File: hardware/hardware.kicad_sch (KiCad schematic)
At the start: 30 parts, among them J2 AudioPlug4, J3 USB_C_Receptacle_USB2.0, J4 AudioPlug4, SW1 SW_Push, SW2 SW_Push, SW3 SW_Push, SW4 SW_Push, SW5 SW_Push, SW6 SW_Push, SW7 SW_Push

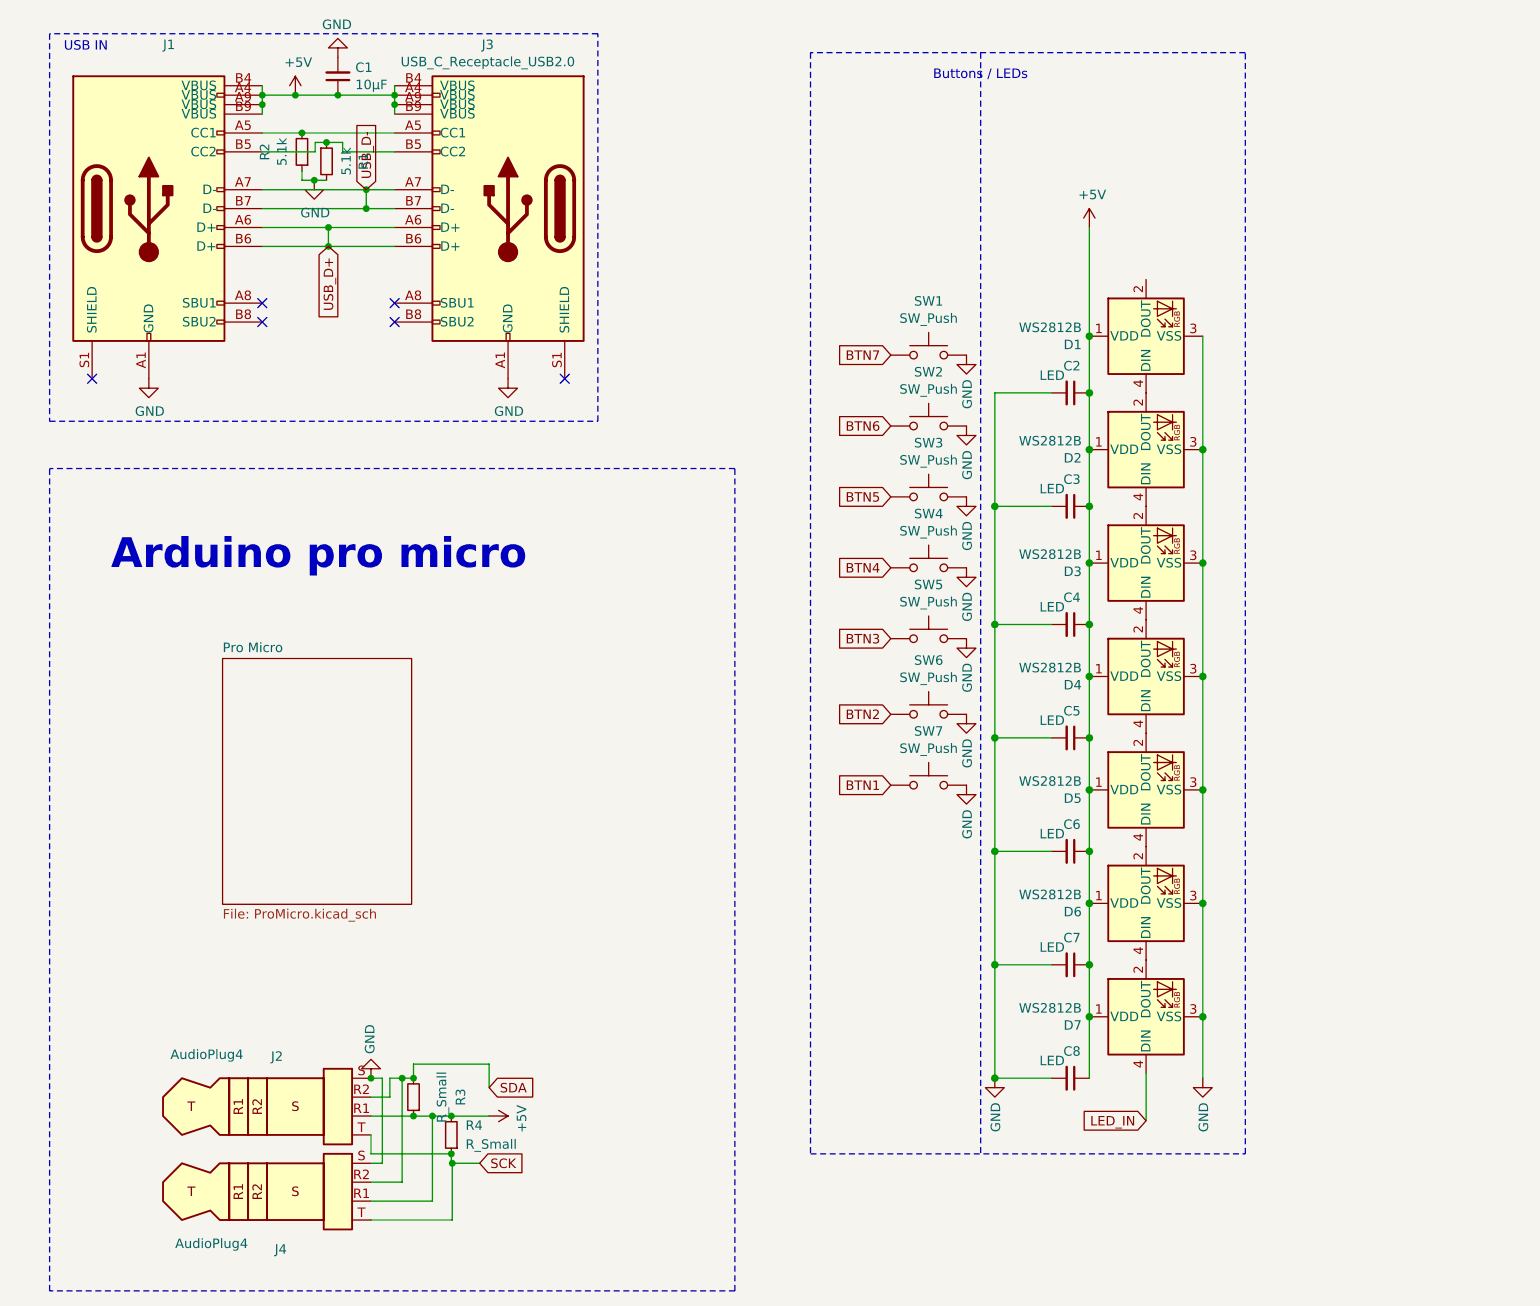
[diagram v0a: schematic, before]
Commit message: finish routing
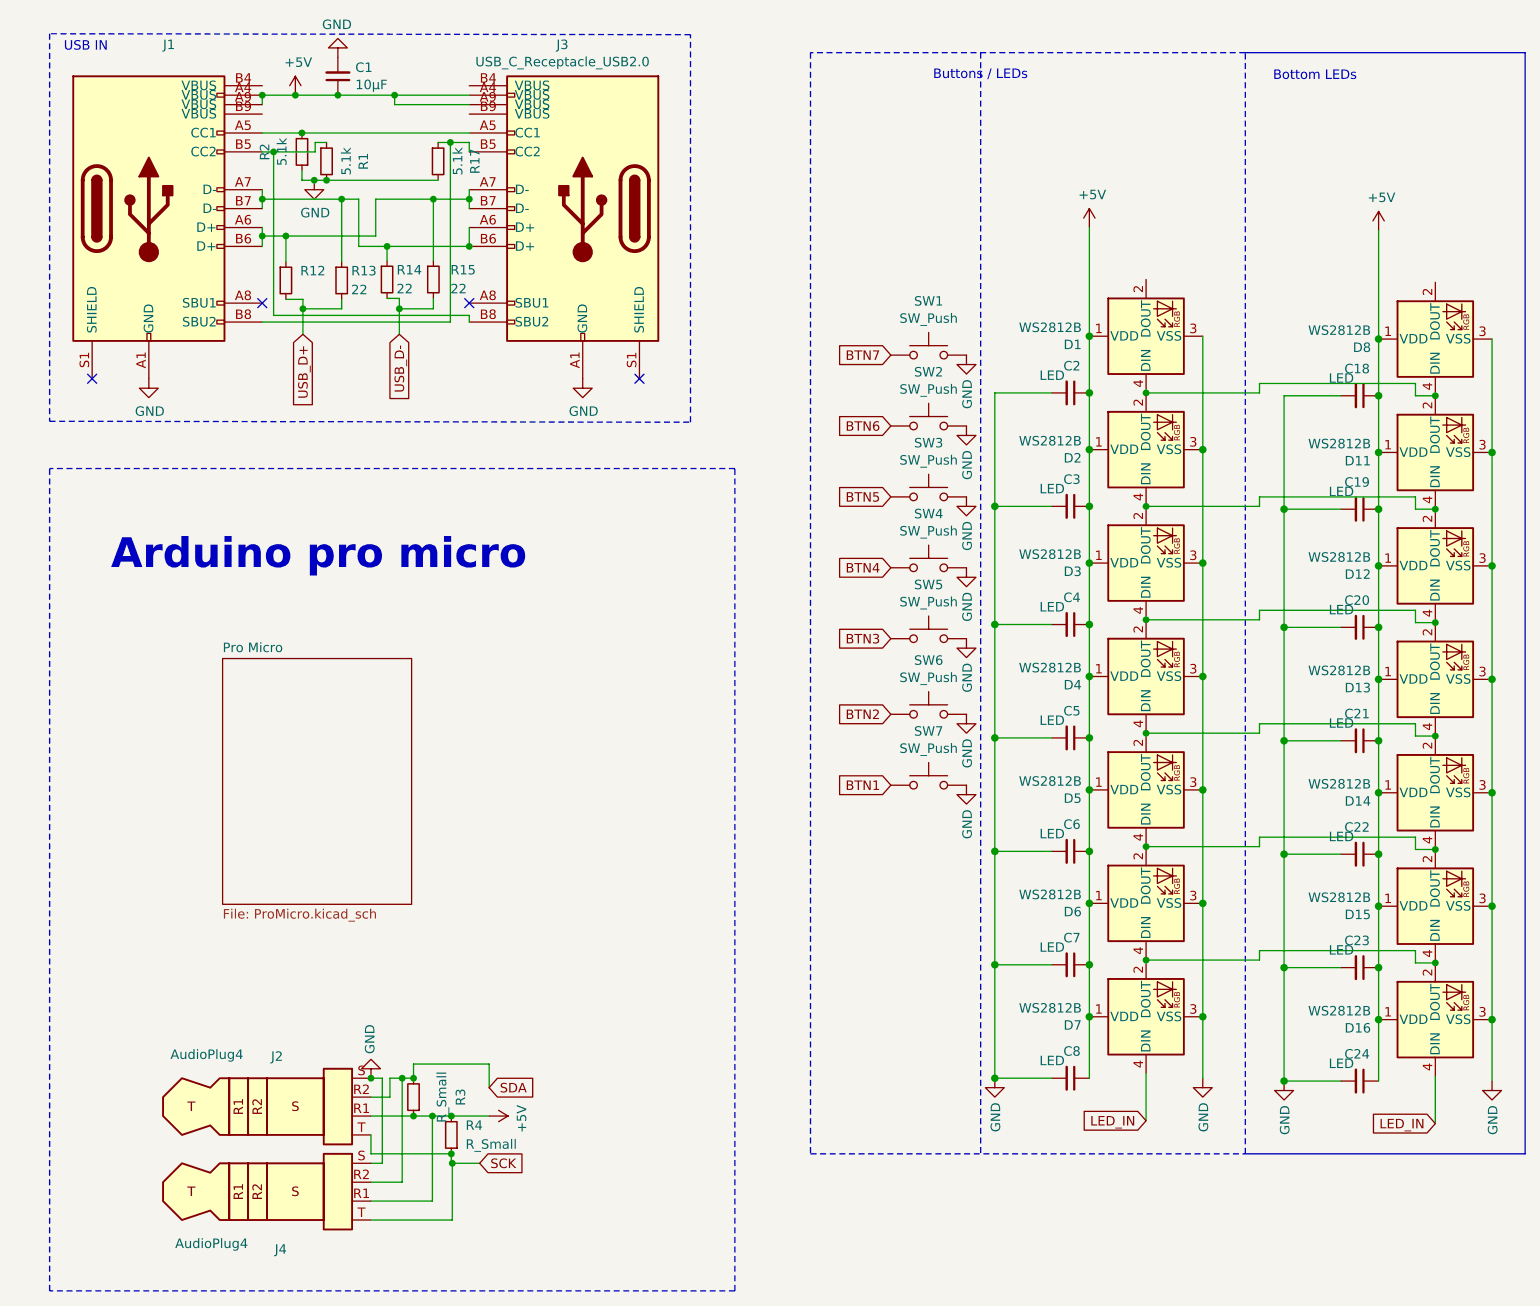
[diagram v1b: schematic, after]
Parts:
- added C18, C19, C20, C21, C22, C23, C24: LED, Capacitor_SMD:C_0603_1608Metric_Pad1.08x0.95mm_HandSolder, symbol Device:C_Small
- added D11, D12, D13, D14, D15, D16, D8: WS2812B, Library:LED_WS2812B_PLCC4_2.2x2.2mm, symbol LED:WS2812B
- added R12: (no value), symbol Device:R_Small
- added R13, R14, R15: 22, Resistor_SMD:R_0603_1608Metric_Pad0.98x0.95mm_HandSolder, symbol Device:R_Small
- added R17: 5.1k, Resistor_SMD:R_0603_1608Metric_Pad0.98x0.95mm_HandSolder, symbol Device:R_Small
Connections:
- net +5V: now also C18.1, C19.1, C20.1, C21.1, C22.1, C23.1, C24.1, D11.1 (VDD), D12.1 (VDD), D13.1 (VDD), D14.1 (VDD), D15.1 (VDD), D16.1 (VDD), D8.1 (VDD); no longer J1.B4 (VBUS), J1.B9 (VBUS), J3.B4 (VBUS), J3.B9 (VBUS)
- net GND: now also C18.2, C19.2, C20.2, C21.2, C22.2, C23.2, C24.2, D11.3 (VSS), D12.3 (VSS), D13.3 (VSS), D14.3 (VSS), D15.3 (VSS), D16.3 (VSS), D8.3 (VSS), R17.2
- net LED_IN: now also D16.4 (DIN)
- net USB_D+: now also R12.2, R13.2; no longer J1.A6 (D+), J1.B6 (D+), J3.A6 (D+), J3.B6 (D+)
- net USB_D-: now also R14.2, R15.2; no longer J1.A7 (D-), J1.B7 (D-), J3.A7 (D-), J3.B7 (D-)
- net at J1.B5 (CC2), R1.1: now also J3.B8 (SBU2); no longer J3.B5 (CC2)
- net at J1.B8 (SBU2): now also J3.B5 (CC2), R17.1
- net at D1.4 (DIN), D2.2 (DOUT): now also D11.2 (DOUT), D8.4 (DIN)
- net at D6.4 (DIN), D7.2 (DOUT): now also D15.4 (DIN), D16.2 (DOUT)
- net at D2.4 (DIN), D3.2 (DOUT): now also D11.4 (DIN), D12.2 (DOUT)
- net at D3.4 (DIN), D4.2 (DOUT): now also D12.4 (DIN), D13.2 (DOUT)
- net at D4.4 (DIN), D5.2 (DOUT): now also D13.4 (DIN), D14.2 (DOUT)
- net at D5.4 (DIN), D6.2 (DOUT): now also D14.4 (DIN), D15.2 (DOUT)
- new net: J1.A6 (D+), J1.B6 (D+), J3.A7 (D-), J3.B7 (D-), R12.1, R15.1
- new net: J1.A7 (D-), J1.B7 (D-), J3.A6 (D+), J3.B6 (D+), R13.1, R14.1
- no-connect marks 6 -> 4
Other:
- note added: "Bottom LEDs"
- moved on the sheet: J3
